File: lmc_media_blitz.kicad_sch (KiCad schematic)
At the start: 26 parts, among them J1 Conn_ARM_JTAG_SWD_10, Q1 BSS138, Q2 BSS138, U1 TPS61222DCK, U2 TLV77333PDBVR, U3 LPC804M101JDH20

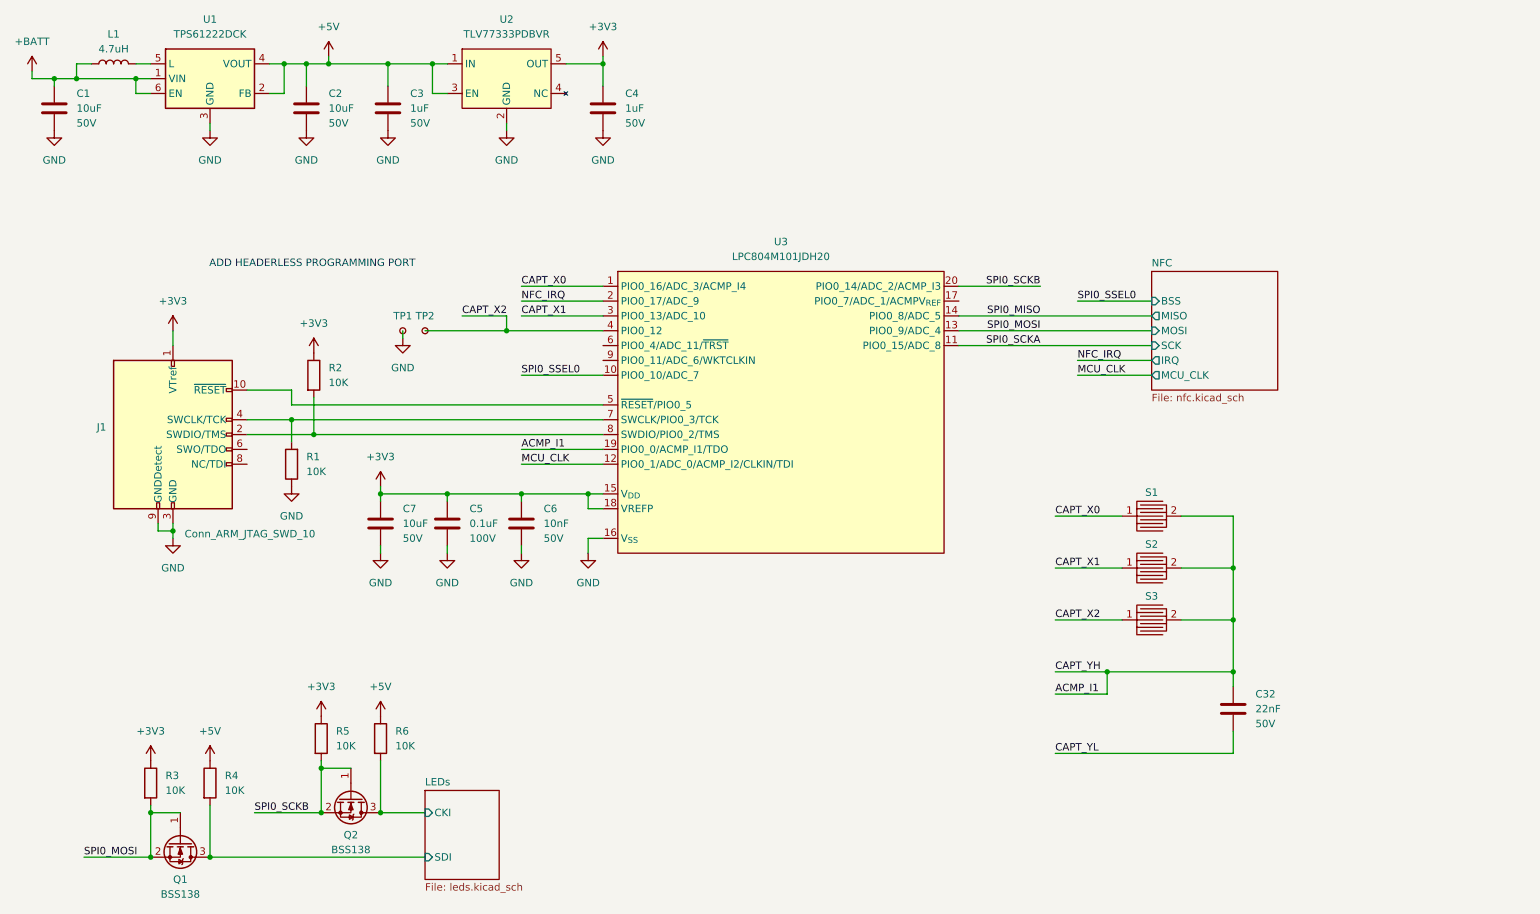
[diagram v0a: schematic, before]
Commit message: Adding some stuf
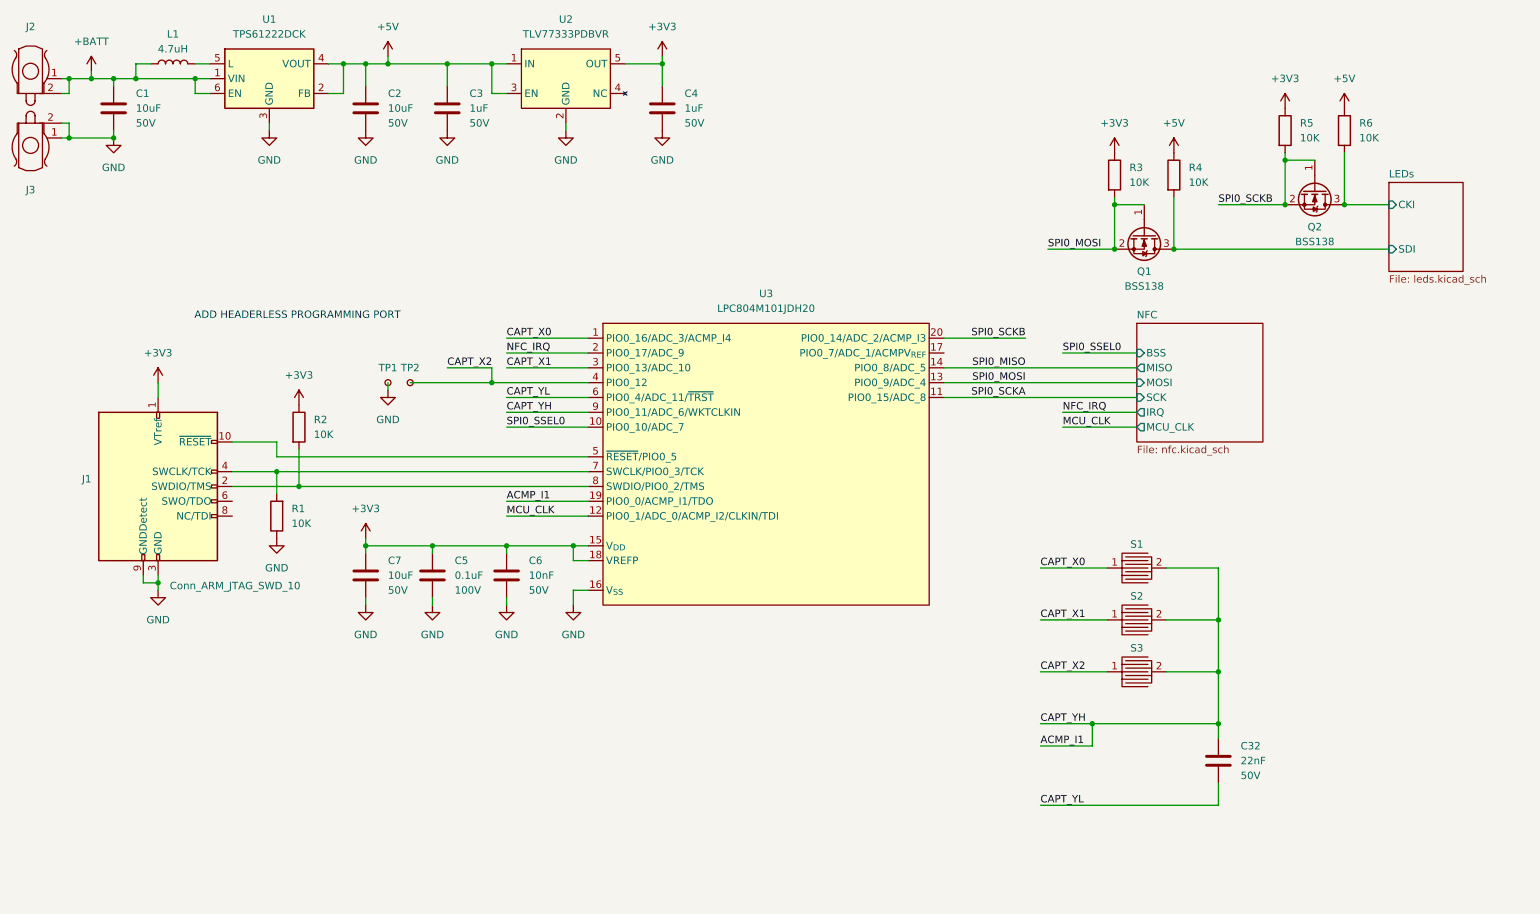
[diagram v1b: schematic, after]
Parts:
- added J2, J3: ~, footprints:Keystone82, symbol parts:Keystone82
- C32: footprint 0805 -> Capacitor_SMD:C_0805_2012Metric
- J1: footprint (none) -> Capacitor_SMD:C_0805_2012Metric
- TP1, TP2: footprint (none) -> TestPoint:TestPoint_Pad_D2.0mm
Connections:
- net +BATT: now also J2.1, J2.2
- net ACMP_I1: now also U3.9 (PIO0_11/ADC_6/WKTCLKIN)
- net CAPT_YL: now also U3.6 (PIO0_4/ADC_11/~{TRST})
- net GND: now also J3.1, J3.2
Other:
- moved on the sheet: C1, C2, C3, C32, C4, C5, C6, C7, J1, L1, Q1, Q2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
